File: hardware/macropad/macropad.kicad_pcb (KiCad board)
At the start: 2 copper layers, 126 x 99.5 mm, 7 parts, among them Q1 SW_Push

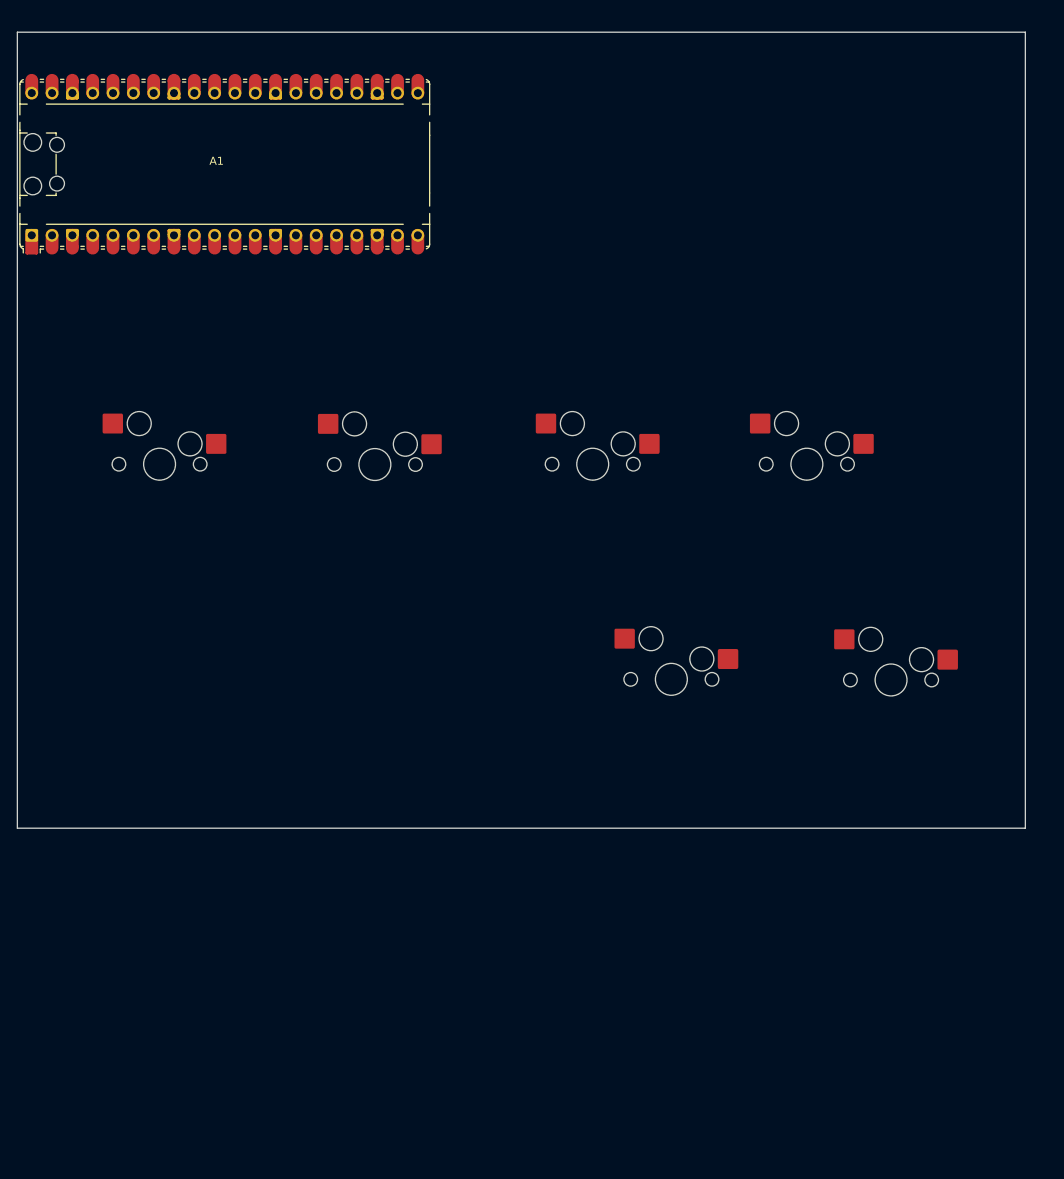
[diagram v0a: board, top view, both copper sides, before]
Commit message: Add Rotary Encoder
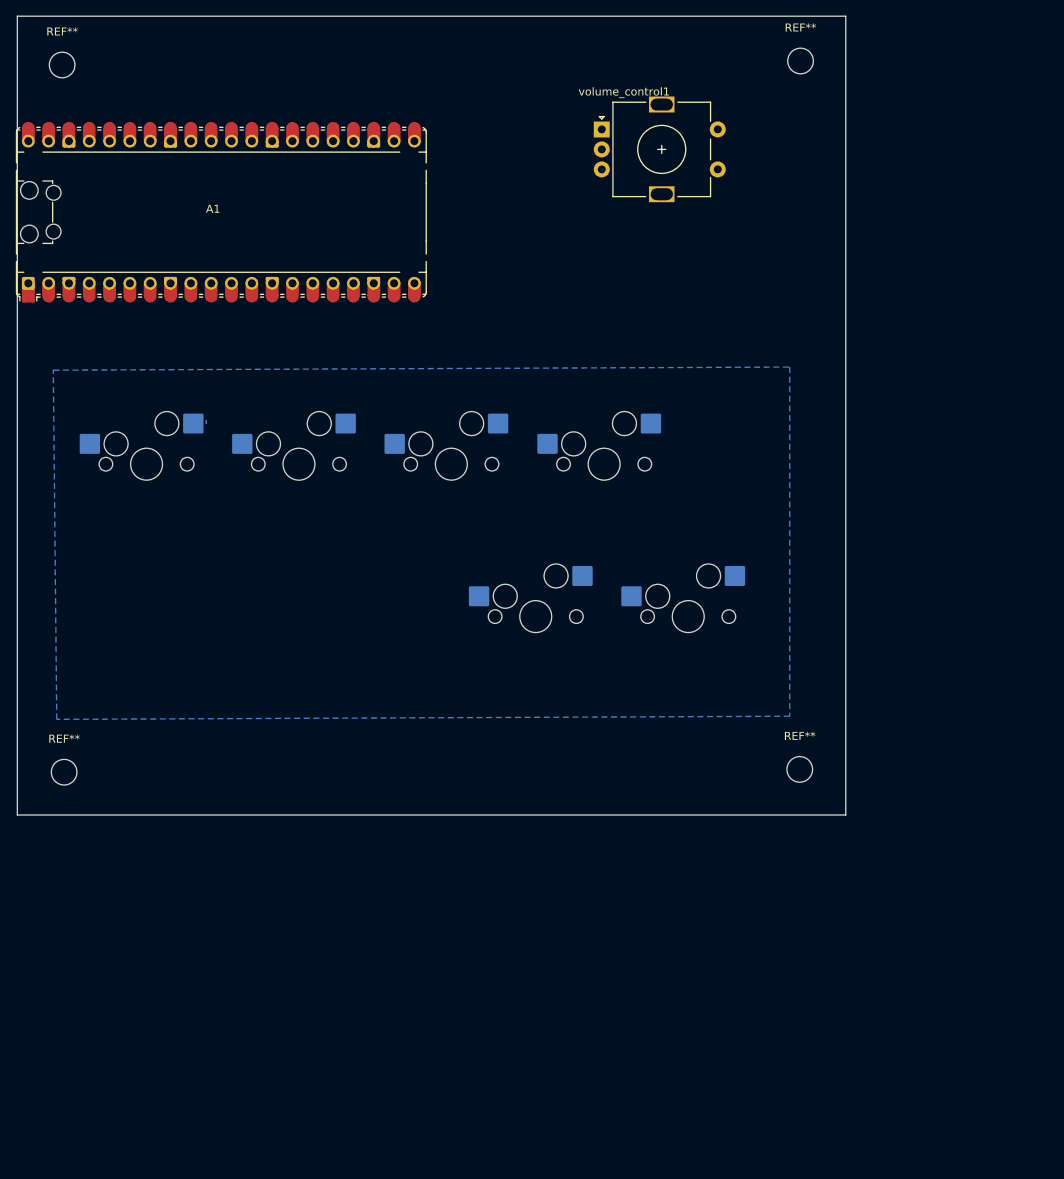
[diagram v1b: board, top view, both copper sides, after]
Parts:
- added REF**: MountingHole_3.2mm_M3, MountingHole:MountingHole_3.2mm_M3, F.Cu at (138.8, 120.7)
- added REF**: MountingHole_3.2mm_M3, MountingHole:MountingHole_3.2mm_M3, F.Cu at (46.9, 121.0)
- added REF**: MountingHole_3.2mm_M3, MountingHole:MountingHole_3.2mm_M3, F.Cu at (46.6, 32.6)
- added REF**: MountingHole_3.2mm_M3, MountingHole:MountingHole_3.2mm_M3, F.Cu at (138.9, 32.1)
- added volume_control1: RotaryEncoder_Switch, Rotary_Encoder:RotaryEncoder_Alps_EC11E-Switch_Vertical_H20mm, F.Cu at (114.0, 40.6)
- D1, E1, F1, Q1, R1, W1: moved to B.Cu
- moved F1 26.6 mm to (124.9, 101.5), turned to 180 degrees
- moved R1 25.3 mm to (114.3, 82.5), turned to 180 degrees
- moved D1 18.7 mm to (105.8, 101.5), turned to 180 degrees
- moved E1 17.7 mm to (95.2, 82.5), turned to 180 degrees
- moved W1 9.49 mm to (76.2, 82.5), turned to 180 degrees
- moved A1 6.02 mm to (66.5, 51.0)
- moved Q1 1.62 mm to (57.1, 82.5), turned to 180 degrees
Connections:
- A1 pad 12: unconnected-(A1-GPIO9-Pad12) -> Net-(A1-GPIO9)
- A1 pad 16: Net-(A1-GPIO12) -> unconnected-(A1-GPIO12-Pad16)
- A1 pad 22: Net-(A1-GPIO17) -> unconnected-(A1-GPIO17-Pad22)
- A1 pad 24: unconnected-(A1-GPIO18-Pad24)_1 -> Net-(A1-GPIO18)
- A1 pad 26: unconnected-(A1-GPIO20-Pad26) -> Net-(A1-GPIO20)
- A1 pad 7: unconnected-(A1-GPIO5-Pad7)_1 -> unconnected-(A1-GPIO5-Pad7)
- D1 pad 1: Net-(A1-GPIO12) -> Net-(A1-GPIO14)
- E1 pad 1: Net-(A1-GPIO13) -> Net-(A1-GPIO9)
- F1 pad 1: Net-(A1-GPIO16) -> Net-(A1-GPIO15)
- Q1 pad 1: Net-(A1-GPIO15) -> unconnected-(A1-GPIO1-Pad2)
- R1 pad 1: Net-(A1-GPIO17) -> Net-(A1-GPIO13)
- W1 pad 1: Net-(A1-GPIO14) -> unconnected-(A1-GPIO5-Pad7)
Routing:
- added copper zone on B.Cu, net GND
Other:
- board size 126 x 99.5 mm -> 103.6 x 99.8 mm

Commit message: Complete Back Copper Routing
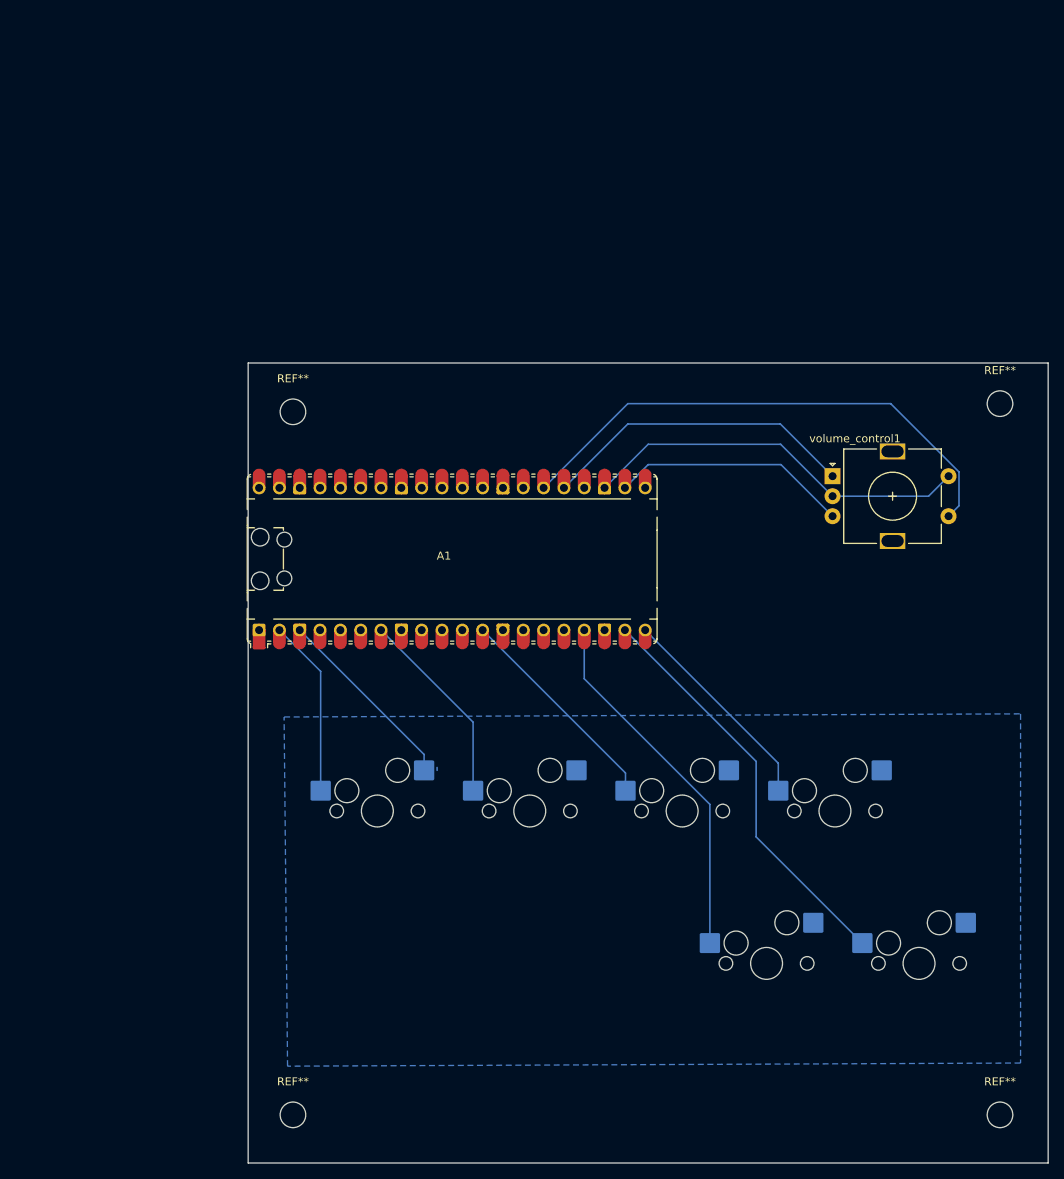
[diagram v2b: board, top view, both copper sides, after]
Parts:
- removed the REF** at (138.8, 120.7)
- removed the REF** at (46.9, 121.0)
- removed the REF** at (138.9, 32.1)
- added REF**: MountingHole_3.2mm_M3, MountingHole:MountingHole_3.2mm_M3, F.Cu at (75.5, 163.8)
- added REF**: MountingHole_3.2mm_M3, MountingHole:MountingHole_3.2mm_M3, F.Cu at (163.8, 74.9)
- added REF**: MountingHole_3.2mm_M3, MountingHole:MountingHole_3.2mm_M3, F.Cu at (163.8, 163.8)
- moved D1 52.1 mm to (134.7, 144.9)
- moved F1 52.1 mm to (153.7, 144.9)
- moved volume_control1 52.1 mm to (142.9, 84.0)
- moved Q1 52.1 mm to (86.0, 125.8)
- moved REF** 52.1 mm to (75.5, 76.0)
- moved A1 52.1 mm to (95.3, 94.3)
- moved E1 52.1 mm to (124.1, 125.8)
- moved R1 52.1 mm to (143.2, 125.8)
- moved W1 52.1 mm to (105.0, 125.8)
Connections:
- A1 pad 21: Net-(A1-GPIO16) -> unconnected-(A1-GPIO16-Pad21)_1
- A1 pad 22: unconnected-(A1-GPIO17-Pad22) -> Net-(A1-GPIO17)
- A1 pad 24: Net-(A1-GPIO18) -> unconnected-(A1-GPIO18-Pad24)_1
- A1 pad 25: unconnected-(A1-GPIO19-Pad25) -> Net-(A1-GPIO19)
- D1 pad 1: Net-(A1-GPIO14) -> Net-(A1-GPIO13)
- F1 pad 1: Net-(A1-GPIO15) -> Net-(A1-GPIO14)
- R1 pad 1: Net-(A1-GPIO13) -> Net-(A1-GPIO15)
- volume_control1 pad A: Net-(A1-GPIO18) -> Net-(A1-GPIO19)
- volume_control1 pad B: Net-(A1-GPIO16) -> Net-(A1-GPIO17)
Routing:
- net GND: track 0.36 -> 73.4 mm
- net Net-(A1-GPIO20): track 0.00 -> 65.9 mm
- net Net-(A1-GPIO14): track 0.00 -> 51.4 mm
- net Net-(A1-GPIO13): track 0.00 -> 45.6 mm
- net Net-(A1-GPIO19): track 0.00 -> 39.6 mm
- net Net-(A1-GPIO17): track 0.00 -> 29.8 mm
- net Net-(A1-GPIO9): track 0.00 -> 27.5 mm
- net Net-(A1-GPIO15): track 0.00 -> 27.0 mm
- net unconnected-(A1-GPIO5-Pad7): track 0.00 -> 24.8 mm
- net unconnected-(A1-GPIO1-Pad2): track 0.00 -> 22.2 mm
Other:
- board size 103.6 x 99.8 mm -> 100 x 100 mm
